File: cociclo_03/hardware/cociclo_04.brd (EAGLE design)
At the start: 42.2 x 43.9 mm, 15 parts

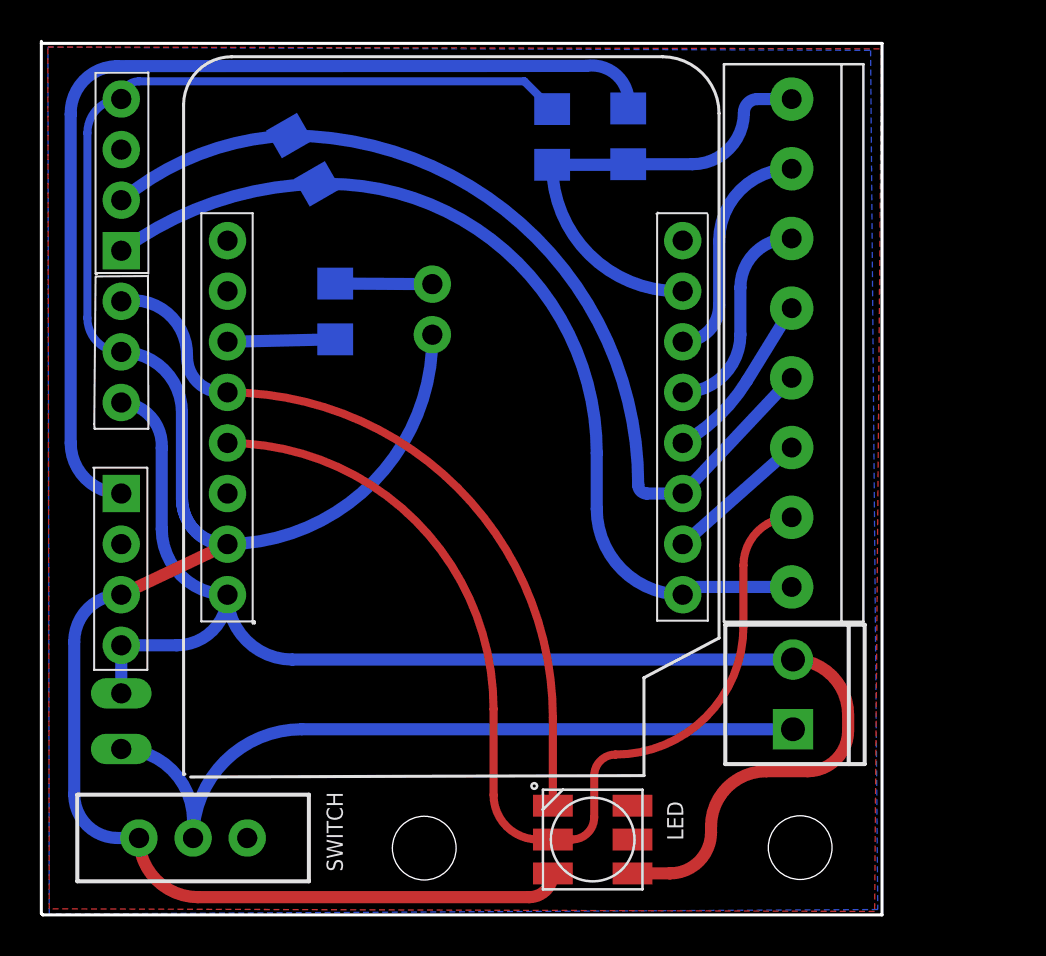
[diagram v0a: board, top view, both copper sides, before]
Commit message: début de la version 05 et fichiers grb
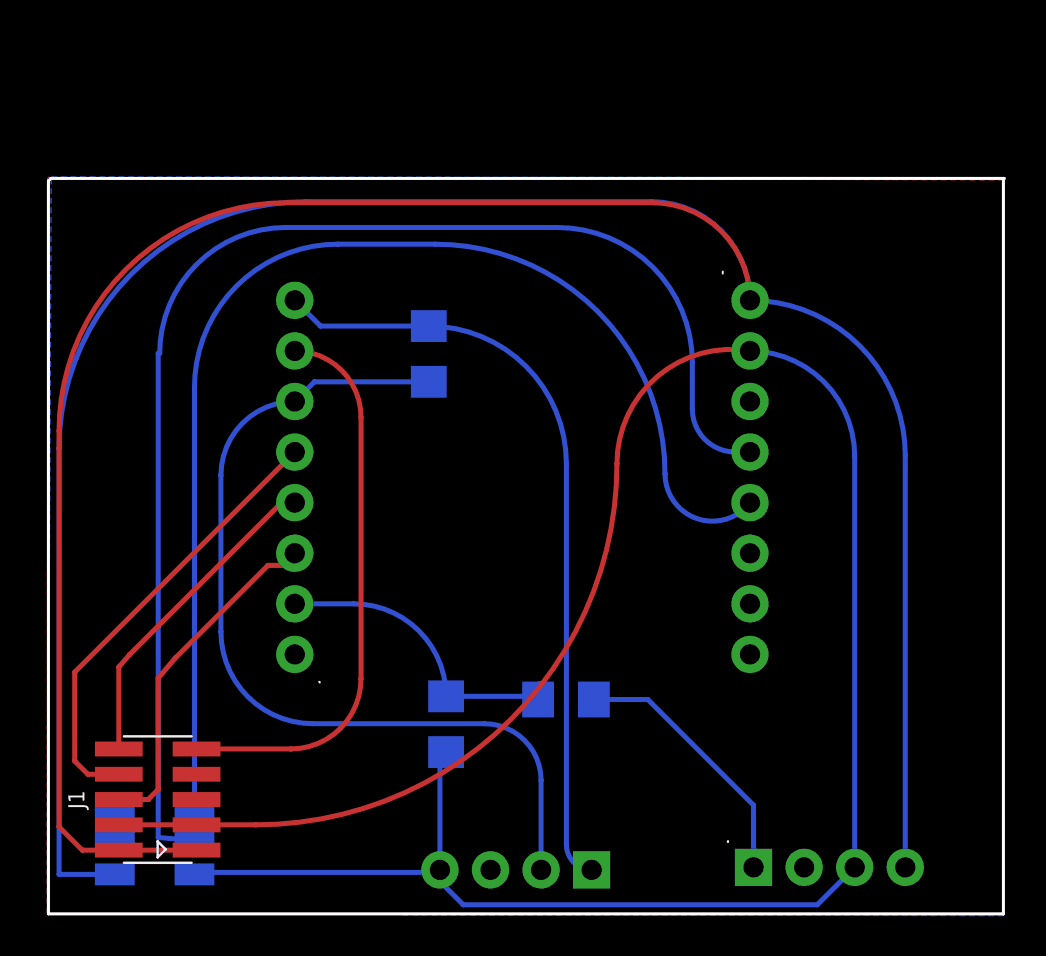
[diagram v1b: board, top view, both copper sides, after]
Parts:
- removed DEL: (no value), SparkFun-Connectors:1X03
- removed JP3: (no value), adafruit:1X08-3.5MM
- removed JP6: (no value), SparkFun-Connectors:SCREWTERMINAL-3.5MM-2
- removed JSPEAKER: (no value), SparkFun-Connectors:1X02
- removed PWR: (no value), SparkFun-Connectors:1X02_LOCK_LONGPADS
- removed R3: 100 ohms, SparkFun-Resistors:1206
- removed SWITCH: (no value), SparkFun-Electromechanical:SWITCH-SPDT_KIT
- added J1: PMS7003, Board-to-Board (rev18a):621X1021021
- moved DHT11 39.0 mm to (27.4, 2.26), turned to 0 degrees
- moved MQ-7 36.9 mm to (35.5, 2.39), turned to 180 degrees
- moved JP2 30.1 mm to (35.3, 30.9), turned to 270 degrees
- moved R1 30.0 mm to (20.1, 9.58), turned to 90 degrees
- moved JP1 28.5 mm to (12.5, 13.1), turned to 90 degrees
- moved R2 28.5 mm to (26.1, 10.8), turned to 0 degrees
- moved LED 22.0 mm to (5.44, 3.73), flipped to the bottom
- moved R6 11.6 mm to (19.2, 28.2), turned to 270 degrees
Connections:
- removed net GPIO12: JP2.6, R3.1
- removed net N$11: JP1.5, JP3.5
- removed net N$12: JP1.4, JP3.6
- removed net N$13: JP1.3, JP3.7
- removed net N$4: JSPEAKER.1, R3.2
- removed net N$8: JP1.7, JP3.3
- removed net N$9: JP6.1, PWR.2, SWITCH.2
- new net 10SET: J1.9, JP1.7
- new net 5RESET: J1.6, JP1.3
- new net 7RX: J1.8, JP1.5
- new net 9TX: J1.10, JP1.4
- net +5V: now also J1.1, J1.2; no longer DEL.3, JP6.2, PWR.1
- net ADC: no longer JP3.8
- net CH_PD: no longer JP3.1
- net D2: no longer DEL.1
- net GND: now also J1.3, J1.4; no longer DEL.2, JSPEAKER.2, SWITCH.3
- net GPIO14: no longer JP3.4
- net N$10: no longer JP3.2
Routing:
- net +5V: track 69.0 -> 166.5 mm
- net N$9: track 38.4 -> 0.00 mm
- net MQ7ANALOG: track 50.1 -> 13.3 mm
- net 10SET: track 0.00 -> 27.6 mm
- net 7RX: track 0.00 -> 22.6 mm
- net D2: track 34.6 -> 56.9 mm
- net 5RESET: track 0.00 -> 17.3 mm
- net 9TX: track 0.00 -> 16.4 mm
- net N$10: track 48.8 -> 64.5 mm
- net N$13: track 11.0 -> 0.00 mm
- net N$12: track 10.1 -> 0.00 mm
- net N$11: track 8.77 -> 0.00 mm
- net ADC: track 23.6 -> 15.5 mm
- net N$8: track 7.31 -> 0.00 mm
- net CH_PD: track 44.6 -> 38.5 mm
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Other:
- board size 42.2 x 43.9 mm -> 48 x 36.9 mm
- board text removed: "0.1k"
- board text removed: "5V"
- board text removed: "SPK"
